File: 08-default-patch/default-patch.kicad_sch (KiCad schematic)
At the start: 24 parts

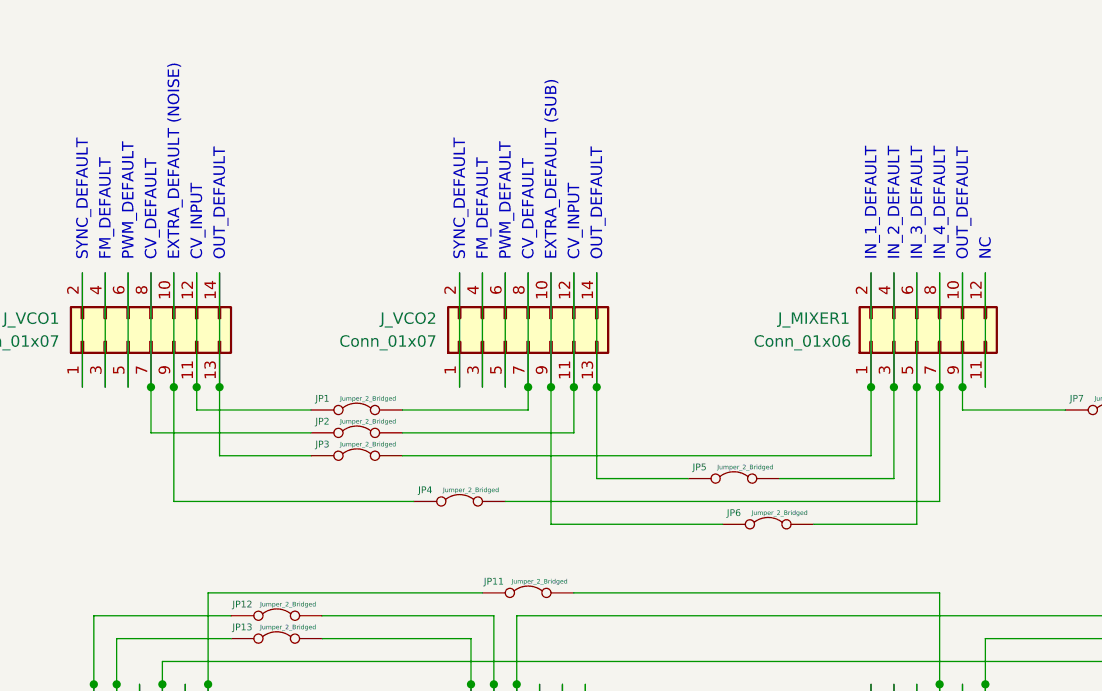
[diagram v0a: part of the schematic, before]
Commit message: Reverted default patch
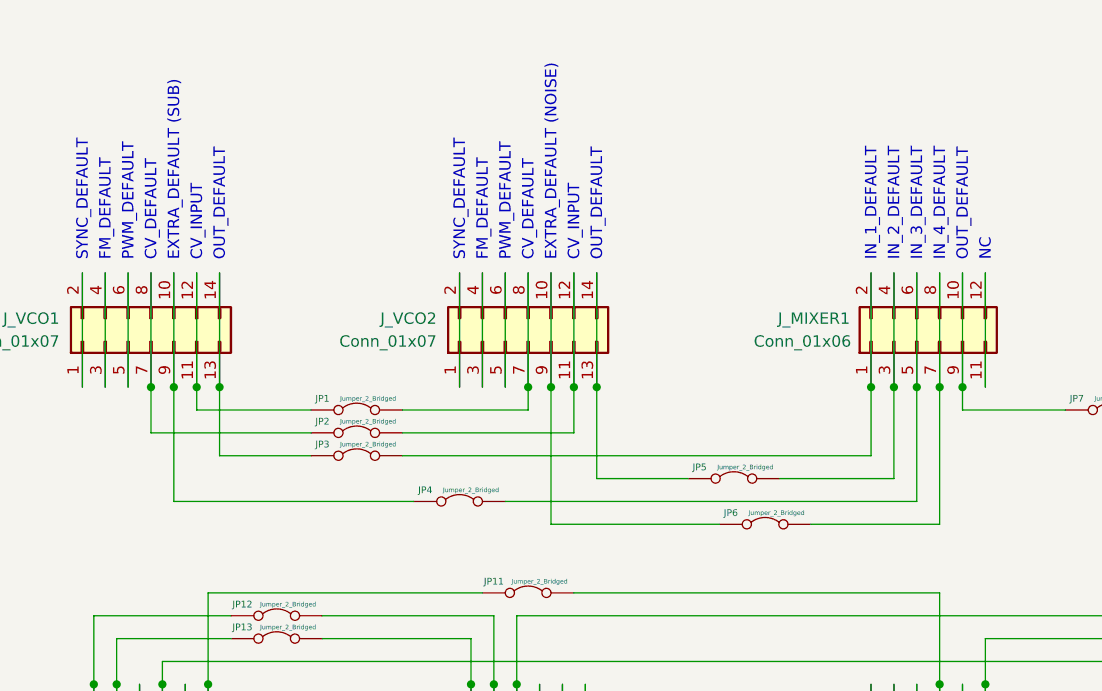
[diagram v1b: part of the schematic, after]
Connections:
- net at J_MIXER1.7 (Pin_7), J_MIXER1.8 (Pin_8): now also JP6.2 (B); no longer JP4.2 (B)
- net at J_MIXER1.5 (Pin_5), J_MIXER1.6 (Pin_6): now also JP4.2 (B); no longer JP6.2 (B)
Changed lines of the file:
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@@
 		)
 	)
-	(text "EXTRA_DEFAULT (SUB)"
+	(text "EXTRA_DEFAULT (NOISE)"
 		(exclude_from_sim no)
 		(at 121.92 63.5 90)
@@
 		)
 	)
-	(text "EXTRA_DEFAULT (NOISE)"
+	(text "EXTRA_DEFAULT (SUB)"
 		(exclude_from_sim no)
 		(at 80.01 63.5 90)
@@
 	)
 	(junction
+		(at 82.55 77.47)
+		(diameter 0)
+		(color 0 0 0 0)
+	)
+	(junction
+		(at 170.18 110.49)
+		(diameter 0)
+		(color 0 0 0 0)
+	)
+	(junction
+		(at 78.74 110.49)
+		(diameter 0)
+		(color 0 0 0 0)
+	)
+	(junction
+		(at 77.47 77.47)
+		(diameter 0)
+		(color 0 0 0 0)
+	)
+	(junction
+		(at 115.57 110.49)
+		(diameter 0)
+		(color 0 0 0 0)
+	)
+	(junction
+		(at 85.09 77.47)
+		(diameter 0)
+		(color 0 0 0 0)
+	)
+	(junction
+		(at 80.01 77.47)
+		(diameter 0)
+		(color 0 0 0 0)
+	)
+	(junction
+		(at 157.48 77.47)
+		(diameter 0)
+		(color 0 0 0 0)
+	)
+	(junction
+		(at 205.74 77.47)
+		(diameter 0)
+		(color 0 0 0 0)
+	)
+	(junction
+		(at 73.66 110.49)
+		(diameter 0)
+		(color 0 0 0 0)
+	)
+	(junction
 		(at 162.56 77.47)
 		(diameter 0)
@@
 	)
 	(junction
-		(at 82.55 77.47)
-		(diameter 0)
-		(color 0 0 0 0)
-	)
-	(junction
-		(at 170.18 110.49)
-		(diameter 0)
-		(color 0 0 0 0)
-	)
-	(junction
-		(at 78.74 110.49)
-		(diameter 0)
-		(color 0 0 0 0)
-	)
-	(junction
-		(at 77.47 77.47)
-		(diameter 0)
-		(color 0 0 0 0)
-	)
-	(junction
-		(at 115.57 110.49)
-		(diameter 0)
-		(color 0 0 0 0)
-	)
-	(junction
-		(at 85.09 77.47)
-		(diameter 0)
-		(color 0 0 0 0)
-	)
-	(junction
-		(at 80.01 77.47)
-		(diameter 0)
-		(color 0 0 0 0)
-	)
-	(junction
-		(at 157.48 77.47)
-		(diameter 0)
-		(color 0 0 0 0)
-	)
-	(junction
-		(at 205.74 77.47)
-		(diameter 0)
-		(color 0 0 0 0)
-	)
-	(junction
-		(at 73.66 110.49)
-		(diameter 0)
-		(color 0 0 0 0)
-	)
-	(junction
 		(at 165.1 110.49)
 		(diameter 0)
@@
 	)
 	(junction
+		(at 124.46 77.47)
+		(diameter 0)
+		(color 0 0 0 0)
+	)
+	(junction
+		(at 210.82 77.47)
+		(diameter 0)
+		(color 0 0 0 0)
+	)
+	(junction
+		(at 83.82 110.49)
+		(diameter 0)
+		(color 0 0 0 0)
+	)
+	(junction
+		(at 119.38 77.47)
+		(diameter 0)
+		(color 0 0 0 0)
+	)
+	(junction
 		(at 165.1 77.47)
 		(diameter 0)
@@
 	)
 	(junction
-		(at 124.46 77.47)
-		(diameter 0)
-		(color 0 0 0 0)
-	)
-	(junction
-		(at 210.82 77.47)
-		(diameter 0)
-		(color 0 0 0 0)
-	)
-	(junction
-		(at 83.82 110.49)
-		(diameter 0)
-		(color 0 0 0 0)
-	)
-	(junction
-		(at 119.38 77.47)
-		(diameter 0)
-		(color 0 0 0 0)
-	)
-	(junction
 		(at 121.92 77.47)
 		(diameter 0)
@@
 	(wire
 		(pts
+			(xy 150.7886 92.71) (xy 165.1 92.71)
+		)
+		(stroke
+			(width 0)
+			(type default)
+		)
+	)
+	(wire
+		(pts
 			(xy 83.82 100.33) (xy 114.3 100.33)
 		)
@@
 	(wire
 		(pts
-			(xy 121.92 92.71) (xy 140.97 92.71)
+			(xy 121.92 92.71) (xy 140.6286 92.71)
 		)
 		(stroke
@@
 	(wire
 		(pts
-			(xy 116.84 90.17) (xy 165.1 90.17)
+			(xy 116.84 90.17) (xy 162.56 90.17)
 		)
 		(stroke
@@
 	(wire
 		(pts
-			(xy 162.56 92.71) (xy 162.56 77.47)
-		)
-		(stroke
-			(width 0)
-			(type default)
-		)
-	)
-	(wire
-		(pts
 			(xy 205.74 105.41) (xy 205.74 91.44)
 		)
@@
 	(wire
 		(pts
+			(xy 162.56 90.17) (xy 162.56 77.47)
+		)
+		(stroke
+			(width 0)
+			(type default)
+		)
+	)
+	(wire
+		(pts
 			(xy 189.23 80.01) (xy 203.2 80.01)
 		)
@@
 	(wire
 		(pts
+			(xy 165.1 92.71) (xy 165.1 77.47)
+		)
+		(stroke
+			(width 0)
+			(type default)
+		)
+	)
+	(wire
+		(pts
 			(xy 119.38 64.77) (xy 119.38 77.47)
 		)
@@
 	(wire
 		(pts
-			(xy 151.13 92.71) (xy 162.56 92.71)
-		)
-		(stroke
-			(width 0)
-			(type default)
-		)
-	)
-	(wire
-		(pts
 			(xy 203.2 80.01) (xy 203.2 77.47)
 		)
@@
 		(pts
 			(xy 127 64.77) (xy 127 77.47)
-		)
-		(stroke
-			(width 0)
-			(type default)
-		)
-	)
-	(wire
-		(pts
-			(xy 165.1 90.17) (xy 165.1 77.47)
 		)
 		(stroke
@@
 	(symbol
 		(lib_id "Jumper:Jumper_2_Bridged")
-		(at 146.05 92.71 0)
+		(at 145.7086 92.71 0)
 		(unit 1)
 		(exclude_from_sim no)
@@
 		(dnp no)
 		(property "Reference" "JP6"
-			(at 142.24 91.44 0)
+			(at 141.8986 91.44 0)
 			(effects
 				(font
@@
 		)
 		(property "Value" "Jumper_2_Bridged"
-			(at 147.32 91.44 0)
+			(at 146.9786 91.44 0)
 			(effects
 				(font
@@
 		)
 		(property "Footprint" "Jumper:SolderJumper-2_P1.3mm_Bridged_RoundedPad1.0x1.5mm"
-			(at 146.05 92.71 0)
+			(at 145.7086 92.71 0)
 			(effects
 				(font
@@
 		)
 		(property "Datasheet" "~"
-			(at 146.05 92.71 0)
+			(at 145.7086 92.71 0)
 			(effects
 				(font
@@
 		)
 		(property "Description" "Jumper, 2-pole, closed/bridged"
-			(at 146.05 92.71 0)
+			(at 145.7086 92.71 0)
 			(effects
 				(font
@@
 		)
 		(property "Part No." ""
-			(at 146.05 92.71 0)
+			(at 145.7086 92.71 0)
 			(effects
 				(font
@@
 		)
 		(property "Part URL" ""
-			(at 146.05 92.71 0)
+			(at 145.7086 92.71 0)
 			(effects
 				(font
@@
 		)
 		(property "Vendor" ""
-			(at 146.05 92.71 0)
+			(at 145.7086 92.71 0)
 			(effects
 				(font
@@
 		)
 		(property "LCSC" ""
-			(at 146.05 92.71 0)
-			(effects
-				(font
+			(at 145.7086 92.71 0)
+			(effects
+				(font
